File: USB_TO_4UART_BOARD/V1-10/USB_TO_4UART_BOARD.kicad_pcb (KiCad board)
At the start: 2 copper layers, 56 parts, among them J3 SIL1, P1 CONN_4, P2 CONN_4, P3 CONN_4, P4 CONN_4, P5 CONN_4, U1 93C46, U2 LM1117, U3 FT4232-HL, U4 74HC02, U5 74LVCC3245, U6 74LVCC3245, X1 12Mhz

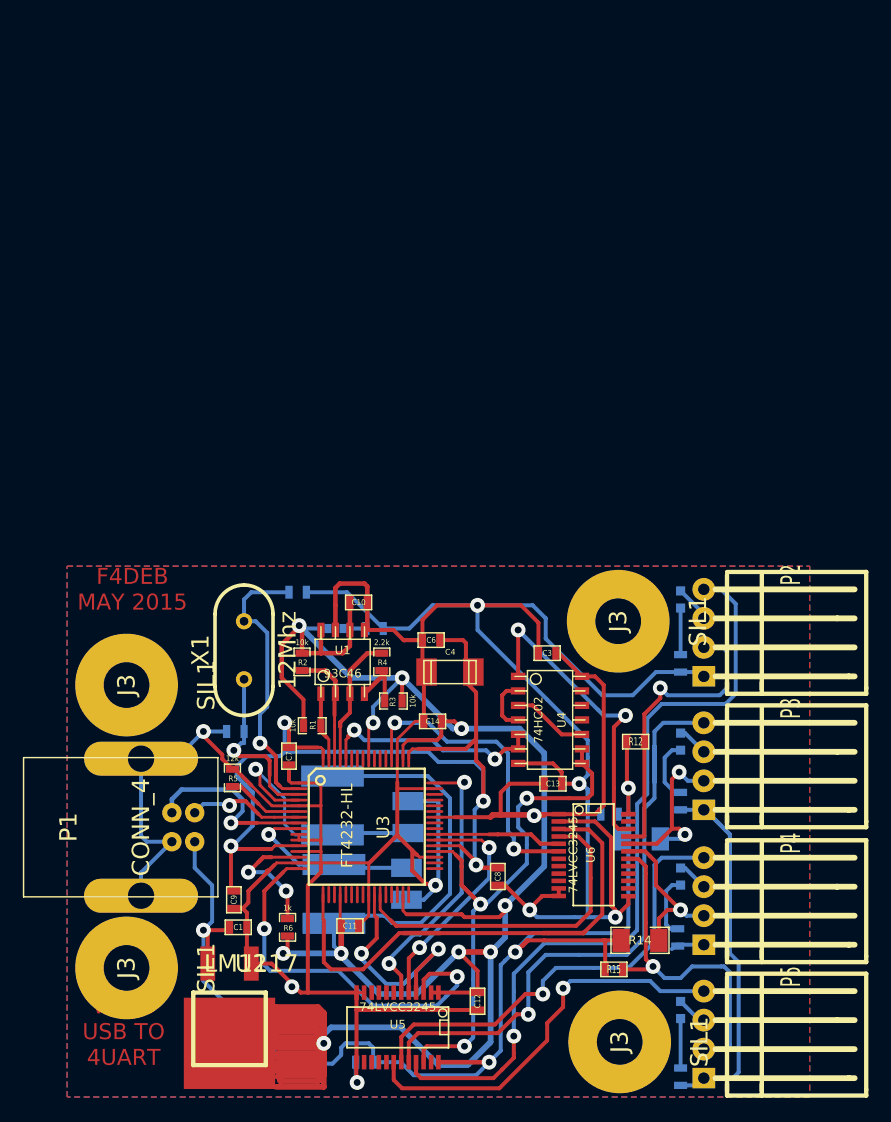
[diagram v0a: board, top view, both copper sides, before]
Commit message: MAJ 2018
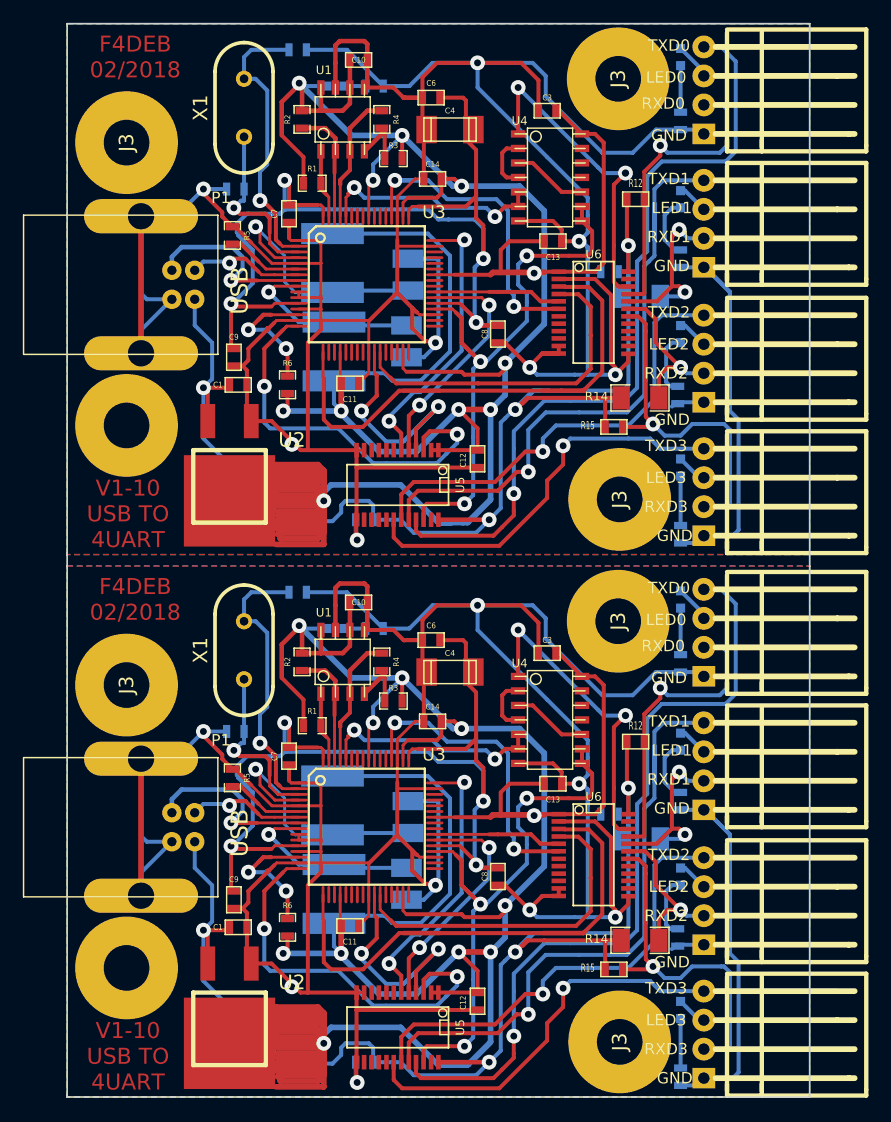
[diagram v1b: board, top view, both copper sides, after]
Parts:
- added C1: 100n, SM0603_Capa, F.Cu at (140.1, 51.8)
- added C10: 100n, SM0603_Capa, F.Cu at (150.6, 23.4)
- added C11: 100n, SM0603_Capa, F.Cu at (149.9, 51.7)
- added C12: 100n, SM0603_Capa, F.Cu at (161.0, 58.3)
- added C13: 100n, SM0603_Capa, F.Cu at (167.6, 39.2)
- added C14: 100n, SM0603_Capa, F.Cu at (157.1, 33.8)
- added C15: 100n, SM0603_Capa, B.Cu at (172.6, 41.9)
- added C16: 100n, SM0603_Capa, B.Cu at (151.1, 63.6)
- added C17: 10uF/10V, SM1210, B.Cu at (154.9, 42.2)
- added C18: 10uF/10V, SM1210, B.Cu at (154.8, 48.0)
- added C2: 27p, SM0603_Capa, B.Cu at (145.3, 22.5)
- added C3: 100n, SM0603_Capa, F.Cu at (167.1, 27.8)
- added C4: 10uF/10V, c_1808, F.Cu at (158.6, 29.5)
- added C5: 27p, SM0603_Capa, B.Cu at (139.8, 34.7)
- added C6: 100n, SM0603_Capa, F.Cu at (157.0, 26.7)
- added C7: 100n, SM0603_Capa, F.Cu at (144.5, 36.8)
- added C8: 100n, SM0603_Capa, F.Cu at (162.8, 47.4)
- added C9: 100n, SM0603_Capa, F.Cu at (139.7, 49.4)
- added D1: +3.3V, LED-0603, B.Cu at (148.6, 25.7)
- added D2: VERT, LED-0603, B.Cu at (178.8, 23.1)
- added D3: VERT, LED-0603, B.Cu at (178.8, 35.6)
- added D4: VERT, LED-0603, B.Cu at (178.8, 47.4)
- added D5: VERT, LED-0603, B.Cu at (178.8, 59.1)
- added J3: SIL1, COLONETTE, F.Cu at (130.3, 55.4)
- added J3: SIL1, COLONETTE, F.Cu at (130.3, 30.6)
- added J3: SIL1, COLONETTE, F.Cu at (173.4, 25.0)
- added J3: SIL1, COLONETTE, F.Cu at (173.5, 61.8)
- added L1: 39uH, c_2220, B.Cu at (148.5, 48.9)
- added L2: 39uH, c_2220, B.Cu at (148.3, 41.1)
- added P1: CONN_4, USB_B, F.Cu at (131.6, 43.1)
- added P2: CONN_4, KK-4-H, F.Cu at (180.8, 22.2)
- added P3: CONN_4, KK-4-H, F.Cu at (180.8, 33.9)
- added P4: CONN_4, KK-4-H, F.Cu at (180.8, 45.7)
- added P5: CONN_4, KK-4-H, F.Cu at (180.8, 57.4)
- added R1: 10k, SM0603_Resistor, F.Cu at (146.6, 34.2)
- added R10: 1k, SM0603_Resistor, B.Cu at (178.6, 52.7)
- added R11: 1k, SM0603_Resistor, B.Cu at (178.8, 64.9)
- added R12: 47k, SM0603_Resistor, F.Cu at (174.9, 35.6)
- added R13: 47k, SM1206, B.Cu at (175.4, 44.1)
- added R14: 47k, SM1206, F.Cu at (175.3, 53.0)
- added R15: 47k, SM0603_Resistor, F.Cu at (173.0, 55.5)
- added R2: 10k, SM0603_Resistor, F.Cu at (145.7, 28.6)
- added R3: 10k, SM0603_Resistor, F.Cu at (153.7, 32.0)
- added R4: 2.2k, SM0603_Resistor, F.Cu at (152.7, 28.6)
- added R5: 12k, SM0603_Resistor, F.Cu at (139.6, 38.7)
- added R6: 1k, SM0603_Resistor, F.Cu at (144.4, 51.8)
- added R7: 470, SM0603_Resistor, B.Cu at (152.0, 25.7)
- added R8: 1k, SM0603_Resistor, B.Cu at (178.8, 28.7)
- added R9: 1k, SM0603_Resistor, B.Cu at (178.8, 40.8)
- added U1: 93C46, so-8, F.Cu at (149.2, 28.6)
- added U2: LM1117, DPAK, F.Cu at (141.2, 55.0)
- added U3: FT4232-HL, TQFP_64, F.Cu at (151.3, 42.9)
- added U4: 74HC02, so-14, F.Cu at (167.4, 33.7)
- added U5: 74LVCC3245, SSOP24, F.Cu at (154.1, 60.6)
- added U6: 74LVCC3245, SSOP24, F.Cu at (171.2, 45.5)
- added X1: 12Mhz, HC-49V, F.Cu at (140.6, 27.6)
- D1: value LED -> +3.3V
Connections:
- P1 pad 5: (no net) -> GND
- P1 pad 6: (no net) -> GND
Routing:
- net GND: track 390.2 -> 804.3 mm, vias 8 -> 16
- net +3.3V: track 383.3 -> 766.7 mm, vias 11 -> 22
- net +5VD: track 115.8 -> 231.6 mm, vias 4 -> 8
- net +1.8V: track 96.1 -> 192.1 mm, vias 4 -> 8
- net /TXD0_5V: track 68.9 -> 137.9 mm, vias 1 -> 2
- net /TXD1_5V: track 56.3 -> 112.6 mm, vias 1 -> 2
- net /SUSPEND: track 50.3 -> 100.6 mm, vias 3 -> 6
- net /RXD0: track 42.6 -> 85.2 mm
- net /TXD2_5V: track 39.8 -> 79.6 mm, vias 1 -> 2
- net /TXD0: track 38.4 -> 76.8 mm, vias 2 -> 4
- net /TXD3_5V: track 35.1 -> 70.3 mm, vias 1 -> 2
- net /RXD3_5V: track 30.2 -> 60.3 mm, vias 1 -> 2
- net /RXD3: track 29.8 -> 59.6 mm, vias 2 -> 4
- net /RXD1: track 29.1 -> 58.1 mm
- net N-0000028: track 27.9 -> 55.9 mm, vias 2 -> 4
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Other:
- board outline added: 65 x 94 mm
- board text added: "F4DEB 02/2018"
- board text added: "GND"
- board text added: "LED0"
- board text added: "LED1"
- board text added: "LED2"
- board text added: "LED3"
- board text added: "RXD0"
- board text added: "RXD1"
- board text added: "RXD2"
- board text added: "RXD3"
- board text added: "TXD0"
- board text added: "TXD1"
- board text added: "TXD2"
- board text added: "TXD3"
- board text added: "UART0"
- board text added: "UART1"
- board text added: "UART2"
- board text added: "UART3"
- board text added: "USB"
- board text removed: "F4DEB MAY 2015"
